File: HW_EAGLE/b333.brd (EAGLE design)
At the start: 80 x 50.5 mm, 153 parts, among them Q1 2N4126, Q2 2N4126, X1 USB MICRO

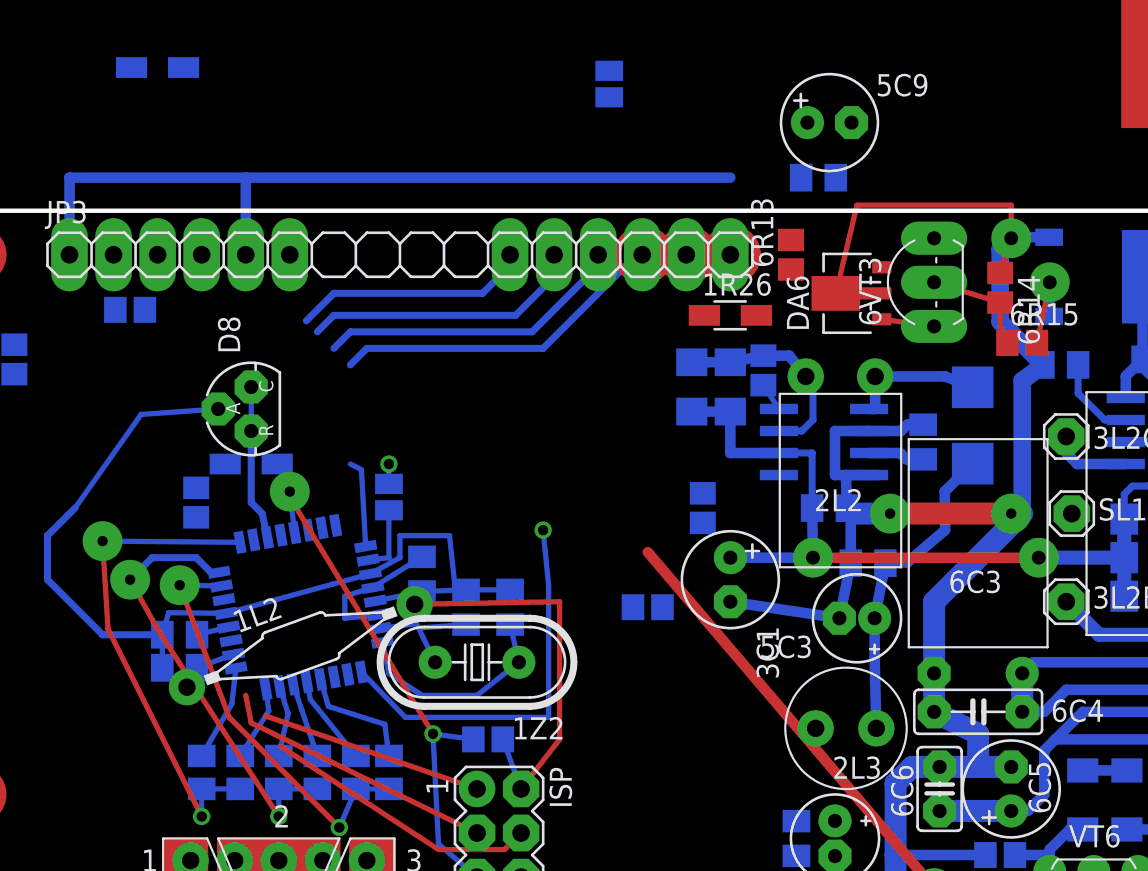
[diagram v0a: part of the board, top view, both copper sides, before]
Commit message: .
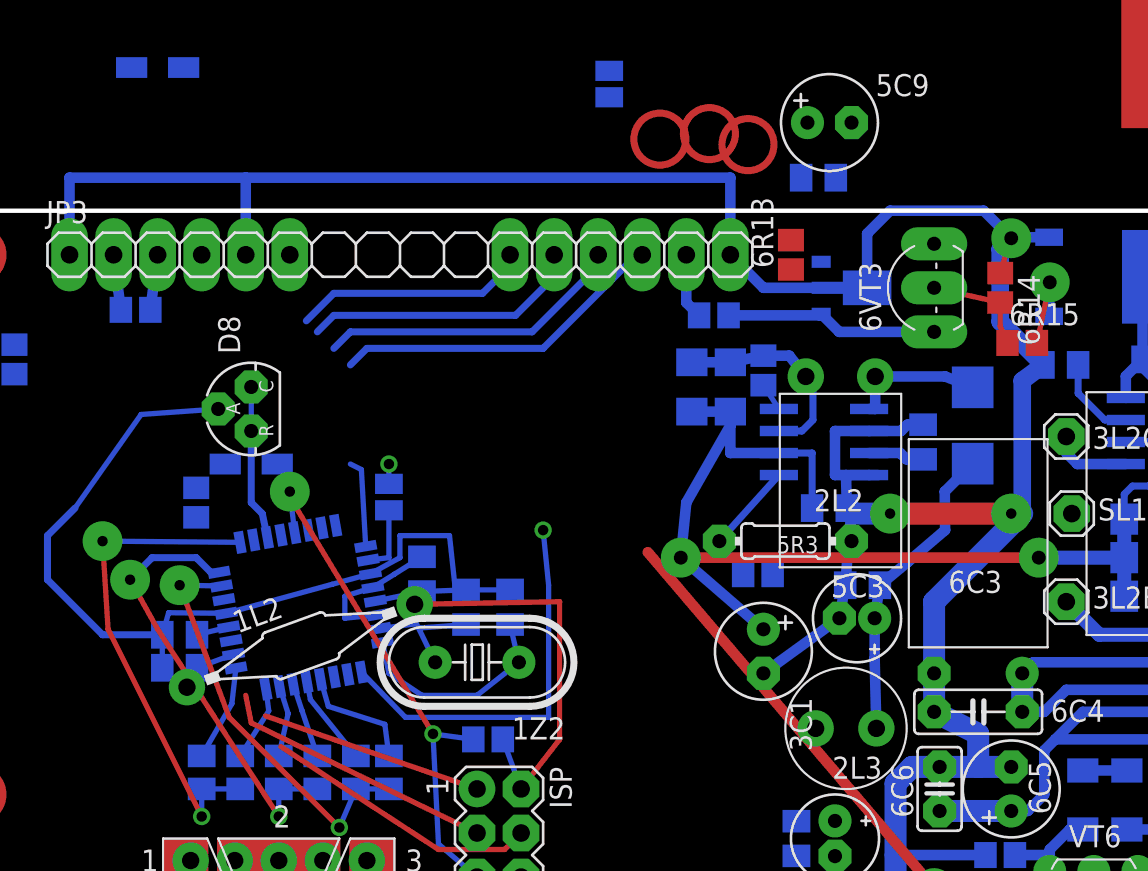
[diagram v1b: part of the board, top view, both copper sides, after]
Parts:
- 1R26: device resistor:R1206W -> resistor:R0805
- 5R3: device resistor:R0805 -> resistor:0204/7
- moved 5R4 6.63 mm to (142.9, 90.8)
- moved 5R3 5.13 mm to (144.5, 92.7), flipped to the top, turned to 180 degrees
- moved 3C1 4.55 mm to (143.2, 86.4)
- moved 5C4 1.31 mm to (148.9, 90.2)
- moved 1R26 0.95 mm to (140.3, 105.7), flipped to the bottom, turned to 180 degrees
- moved 1RC2 0.32 mm to (107.0, 106.0)
- moved 6VT3 0.32 mm to (153.0, 107.3)
- moved DA6 0.32 mm to (148.3, 107.3), flipped to the bottom
- renumbered 1RC2*1 to 1RC3
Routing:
- net V+: track 77.4 -> 92.0 mm
- net +5V/2: track 3.04 -> 15.5 mm
- net GND: track 354.1 -> 360.5 mm
- net N$16: track 0.00 -> 5.13 mm
- net N$61: track 0.00 -> 3.80 mm
- net N$60: track 0.00 -> 3.20 mm
- net N$17: track 18.2 -> 17.7 mm
